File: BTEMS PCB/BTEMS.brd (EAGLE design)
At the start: 44.5 x 63.5 mm, 22 parts

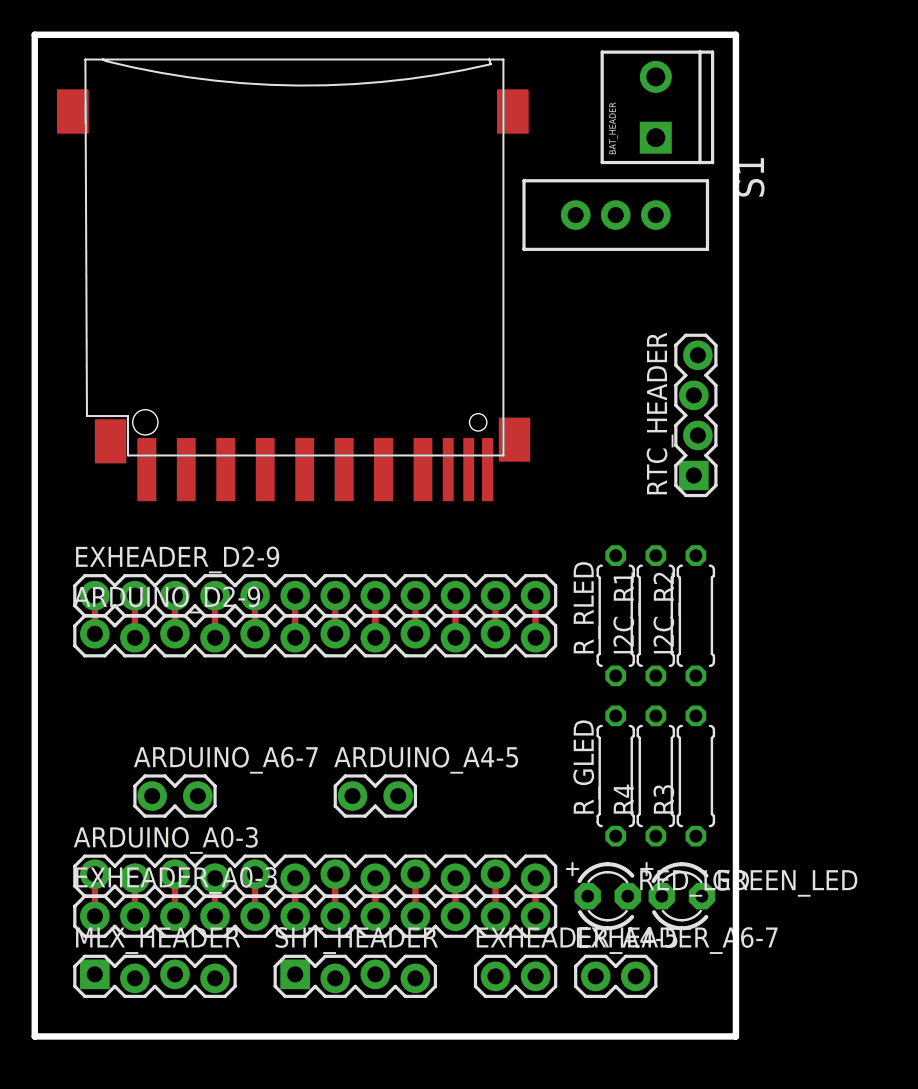
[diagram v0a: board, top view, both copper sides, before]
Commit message: Solidified part position, added BOM
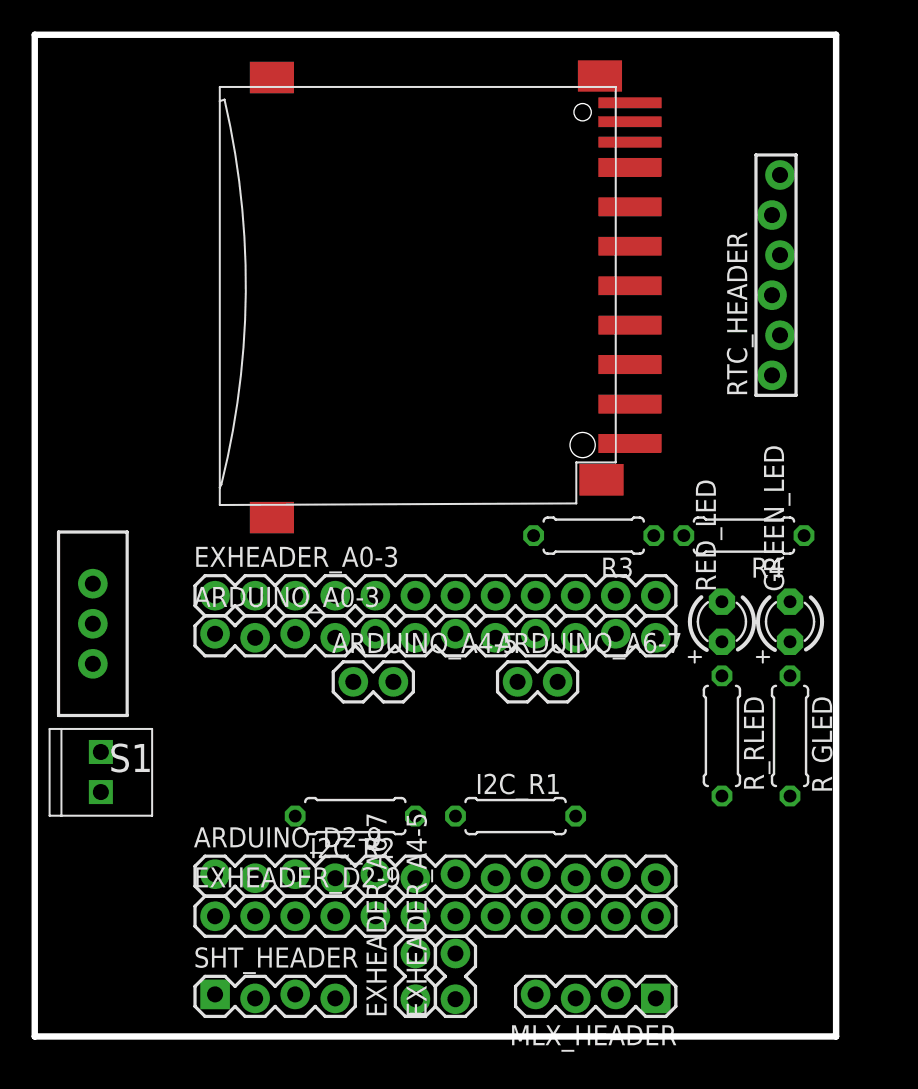
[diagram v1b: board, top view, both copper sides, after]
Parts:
- removed U$1: SDMMC06132, adafruit:06132
- added SDSLOT: SDMMC06132, adafruit:06132
- ARDUINO_A4-5, ARDUINO_A6-7: device SparkFun-Connectors:1X02_LOCK -> SparkFun-Connectors:1X02
- BAT_HEADER: device SparkFun-Connectors:SCREWTERMINAL-3.5MM-2_LOCK -> SparkFun-Connectors:1X02_2.54_SCREWTERM
- EXHEADER_A4-5, EXHEADER_A6-7: device SparkFun-Connectors:1X02 -> SparkFun-Connectors:1X02_LOCK
- I2C_R1, I2C_R2: value (none) -> 2.2k
- RTC_HEADER: device SparkFun-Connectors:1X04_LOCK -> SparkFun-Connectors:1X06_FEMALE_LOCK.010
- moved BAT_HEADER 54.5 mm to (4.19, 15.5)
- moved S1 42.1 mm to (3.68, 26.2), turned to 180 degrees
- moved MLX_HEADER 35.6 mm to (39.4, 2.54), turned to 180 degrees
- moved I2C_R2 25.0 mm to (20.3, 14.0), turned to 180 degrees
- moved ARDUINO_A6-7 24.1 mm to (30.6, 22.5)
- moved EXHEADER_A0-3 21.7 mm to (11.4, 27.9)
- moved EXHEADER_D2-9 21.7 mm to (11.4, 7.62)
- moved RED_LED 18.8 mm to (43.6, 26.3), turned to 90 degrees
- moved GREEN_LED 18.7 mm to (47.9, 26.3), turned to 90 degrees
- moved ARDUINO_A0-3 17.0 mm to (11.4, 25.4)
- moved ARDUINO_D2-9 17.0 mm to (11.4, 10.2)
- moved R3 16.6 mm to (35.4, 31.8), turned to 180 degrees
- moved R4 16.2 mm to (45.0, 31.8), turned to 180 degrees
- moved I2C_R1 15.5 mm to (30.5, 14.0), turned to 0 degrees
- moved EXHEADER_A6-7 11.5 mm to (24.1, 2.54), turned to 90 degrees
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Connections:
- net 3.3V: now also RTC_HEADER.2, RTC_HEADER.5, SDSLOT.4; no longer U$1.4
- net BAT_IN: now also BAT_HEADER.P2; no longer BAT_HEADER.2
- net D11: now also SDSLOT.2; no longer U$1.2
- net D12: now also SDSLOT.7; no longer U$1.7
- net D13: now also SDSLOT.5; no longer U$1.5
- net D4: now also SDSLOT.1; no longer U$1.1
- net GND: now also BAT_HEADER.P1, RTC_HEADER.6, SDSLOT.3, SDSLOT.6, SDSLOT.GP, SDSLOT.GP3; no longer BAT_HEADER.1, U$1.3, U$1.6, U$1.GP, U$1.GP3
- net VCC: no longer RTC_HEADER.2
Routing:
- net RST: track 5.08 -> 0.00 mm
- net GND: track 5.08 -> 0.00 mm
- net RXI: track 2.67 -> 0.00 mm
- net D9: track 2.67 -> 0.00 mm
- net D7: track 2.67 -> 0.00 mm
- net D5: track 2.67 -> 0.00 mm
- net D3: track 2.67 -> 0.00 mm
- net RAW: track 2.67 -> 0.00 mm
- net D13: track 2.67 -> 0.00 mm
- net D11: track 2.67 -> 0.00 mm
- net A3: track 2.67 -> 0.00 mm
- net A1: track 2.67 -> 0.00 mm
- net TXO: track 2.41 -> 0.00 mm
- net D8: track 2.41 -> 0.00 mm
- net D6: track 2.41 -> 0.00 mm
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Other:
- board size 44.5 x 63.5 mm -> 50.8 x 63.5 mm
